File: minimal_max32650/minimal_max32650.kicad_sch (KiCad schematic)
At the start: 108 parts, among them J1 CLP-113-02-G-D-BE, J2 CLP-129-02-G-D-BE, J3 FTSH-105-01-L-DV-K, Q1 50 V, Q2 50 V, U1 ADT75BRMZ, U2 S80KS5122GABHM020, U3 MX25U6432FZNI02, U4 MAX32650GCE+, U5 MAXQ1065GTC+, U6 ADP225ACPZ-R7

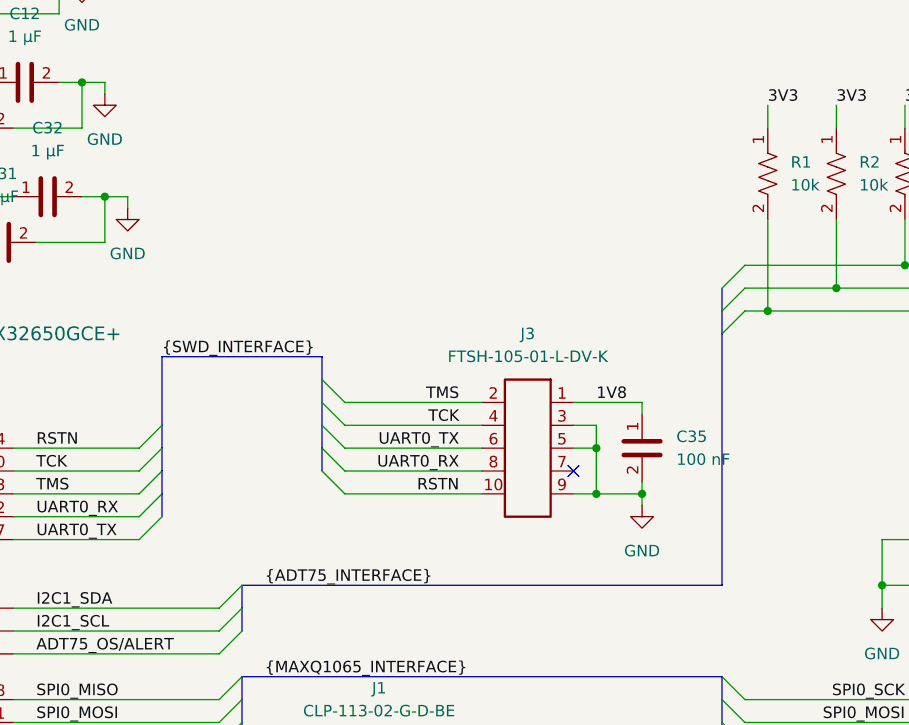
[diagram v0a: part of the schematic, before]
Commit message: development backup
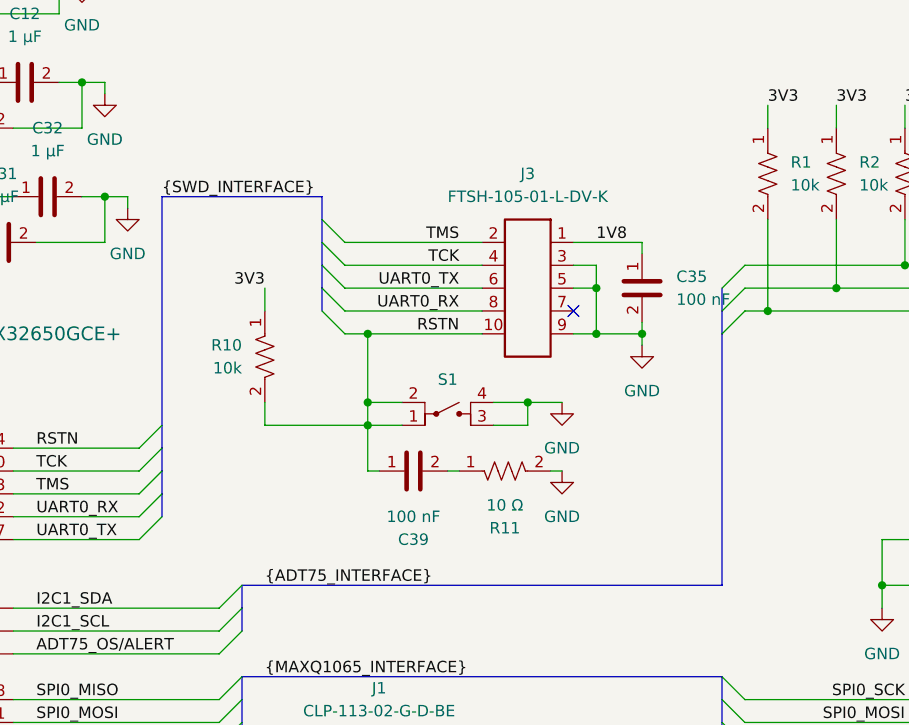
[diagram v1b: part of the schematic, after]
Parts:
- added C39: 100 nF, capacitor_footprints:C_0402_1005Metric, symbol UNITED_CAPACITORS_DATA_BASE:C_GCM155R71H104KE02D
- added R10: 10k, resistor_footprints:R_0402_1005Metric, symbol UNITED_RESISTORS_DATA_BASE:R_ERJ-2RKF1002X
- added R11: 10 Ω, resistor_footprints:R_0402_1005Metric, symbol UNITED_RESISTORS_DATA_BASE:R_ERJ-2RKF10R0X
- added S1: TS21-34-035-BK-160-SMT-TR, tactile_switches_footprints:TS21, symbol UNITED_TACTILE_SWITCHES_DATA_BASE:S_TS21-34-035-BK-160-SMT-TR
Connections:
- net 3V3: now also R10.1
- net GND: now also R11.2, S1.3, S1.4
- net RSTN: now also C39.1, R10.2, S1.1, S1.2
- new net: C39.2, R11.1
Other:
- moved on the sheet: C35, J3
